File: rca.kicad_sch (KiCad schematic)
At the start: 14 parts, among them J4 RCA, U6 OPA1612AxD

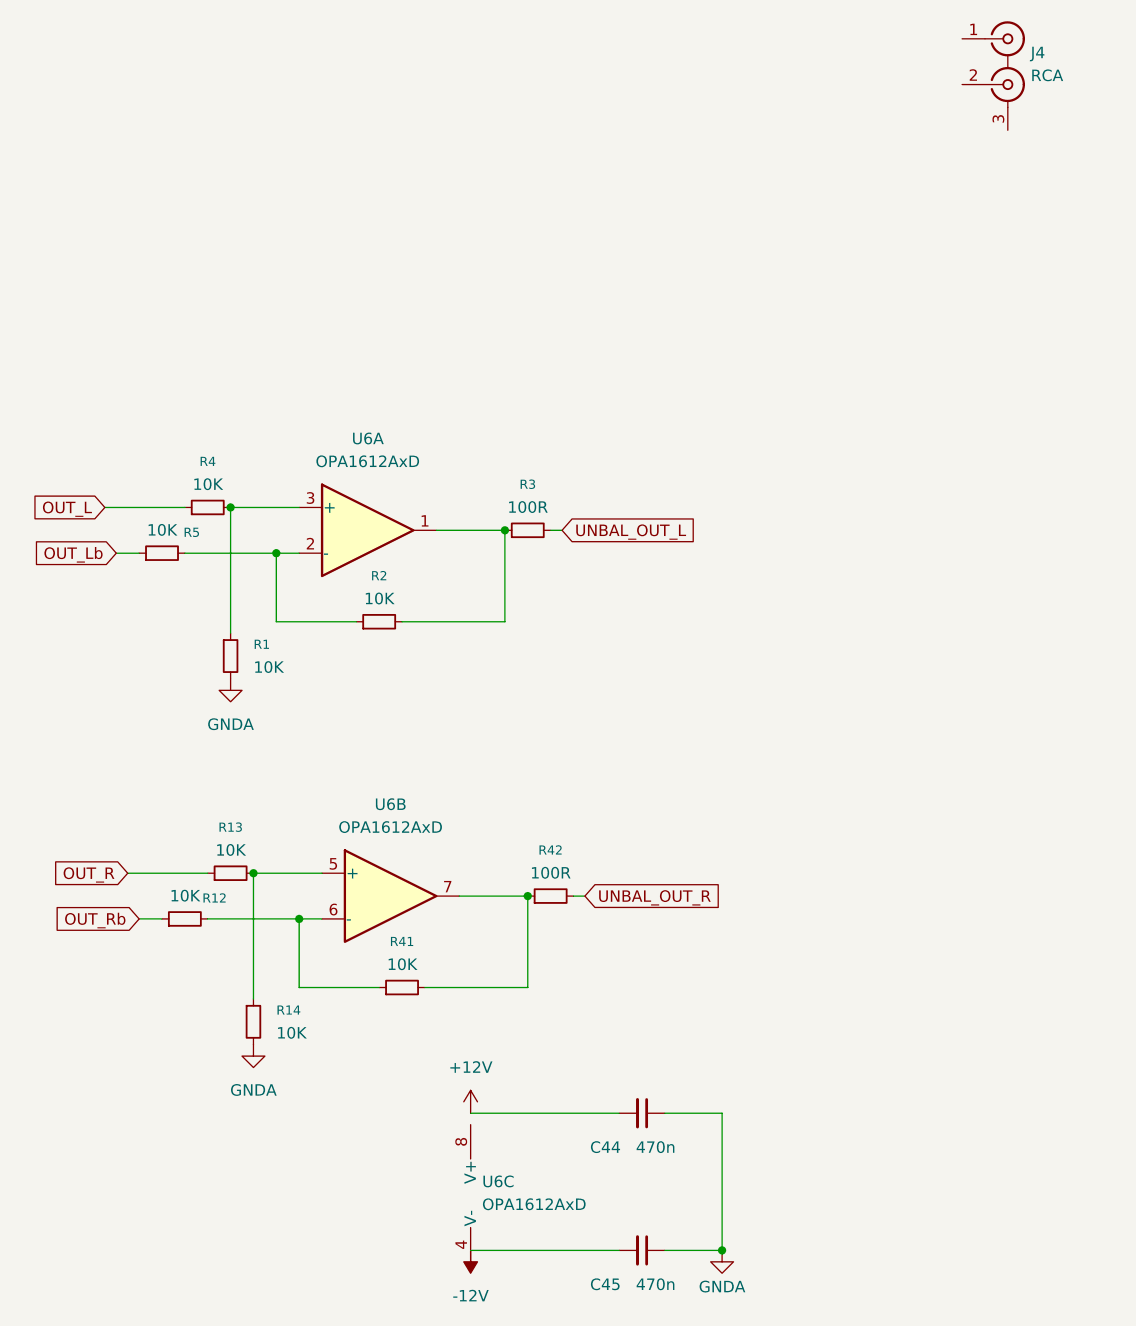
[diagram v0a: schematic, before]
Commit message: add rca
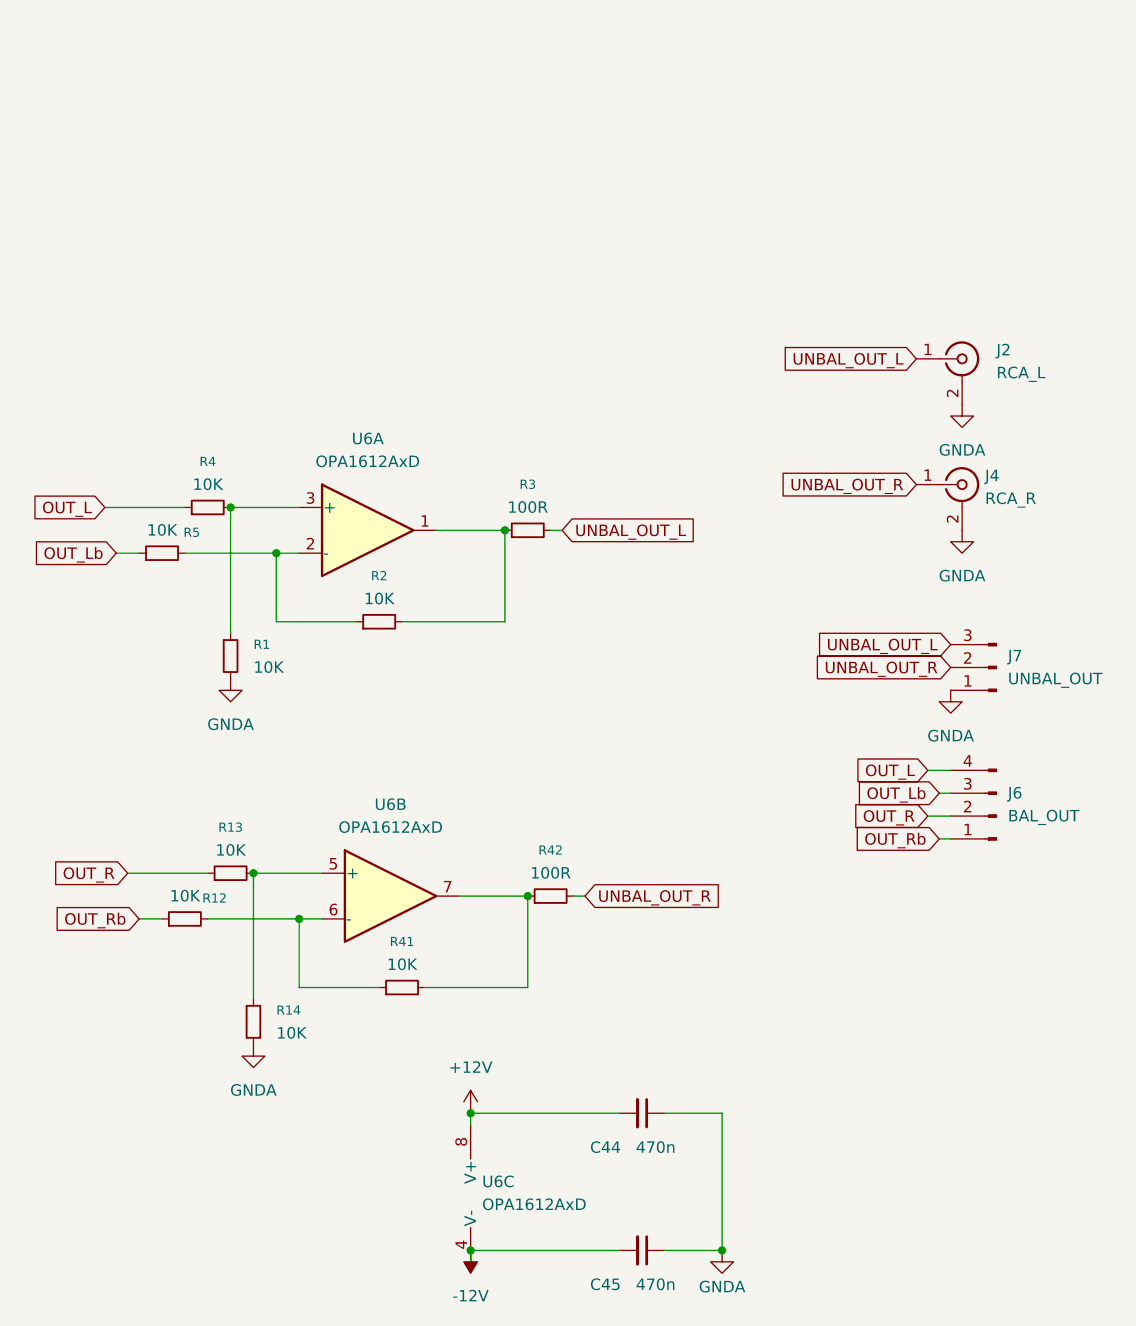
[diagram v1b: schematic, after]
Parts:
- removed J4: RCA, symbol Connector:Conn_Coaxial_x2
- added J2: RCA_L, rca:RCA-105A, symbol Connector:Conn_Coaxial
- added J4: RCA_R, rca:RCA-105A, symbol Connector:Conn_Coaxial
- added J6: BAL_OUT, Connector_PinHeader_2.54mm:PinHeader_1x04_P2.54mm_Vertical, symbol Connector:Conn_01x04_Pin
- added J7: UNBAL_OUT, Connector_PinHeader_2.54mm:PinHeader_1x03_P2.54mm_Vertical, symbol Connector:Conn_01x03_Pin
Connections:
- net +12V: now also U6.8 (V+)
- net -12V: now also U6.4 (V-)
- net GNDA: now also J2.2 (Ext), J4.2 (Ext), J7.1 (Pin_1)
- net OUT_L: now also J6.4 (Pin_4)
- net OUT_Lb: now also J6.3 (Pin_3)
- net OUT_R: now also J6.2 (Pin_2)
- net OUT_Rb: now also J6.1 (Pin_1)
- net UNBAL_OUT_L: now also J2.1 (In), J7.3 (Pin_3)
- net UNBAL_OUT_R: now also J4.1 (In), J7.2 (Pin_2)
